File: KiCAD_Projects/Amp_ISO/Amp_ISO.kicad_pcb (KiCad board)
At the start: 2 copper layers, 0 parts

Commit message: MDver4.0だいたいできた｡絶縁アンプ基板作った｡
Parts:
- added C1: 0.1u, RP_KiCAD_Libs:C1608_WP, B.Cu at (11.5, 6.50)
- added C2: 0.1u, RP_KiCAD_Libs:C1608_WP, B.Cu at (23.0, 4.00)
- added D1: LED, RP_KiCAD_Libs:C1608_WP, B.Cu at (13.0, 13.5)
- added D2: LED, RP_KiCAD_Libs:C1608_WP, B.Cu at (21.0, 13.5)
- added P1: CONN_01X01, Connect:PINTST, F.Cu at (9.00, 11.5)
- added P2: CONN_01X03, RP_KiCAD_Connector:XA_3LC, F.Cu at (21.0, 7.50)
- added P3: CONN_01X01, Connect:PINTST, F.Cu at (8.00, 4.00)
- added P4: CONN_01X01, Connect:PINTST, F.Cu at (8.00, 6.50)
- added PC1: TLP117, RP_KiCAD_Libs:SOIC-5_3.9x4.9mm_Pitch1.27mm, B.Cu at (15.0, 2.50)
- added Q1: MOSFET_N, TO_SOT_Packages_SMD:SOT-23_Handsoldering, B.Cu at (13.0, 9.00)
- added R1: R, RP_KiCAD_Libs:C1608_WP, B.Cu at (9.00, 9.00)
- added R2: R, RP_KiCAD_Libs:C1608_WP, B.Cu at (9.50, 13.5)
- added R3: R, RP_KiCAD_Libs:C1608_WP, B.Cu at (17.5, 13.5)
- added R4: R, RP_KiCAD_Libs:C1608_WP, B.Cu at (14.5, 6.50)
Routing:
- net /GND_POWER: track 0.00 -> 20.5 mm
- net /5V_POWER: track 0.00 -> 20.4 mm
- net /5V_LOGIC: track 0.00 -> 14.7 mm
- net /GND_LOGIC: track 0.00 -> 12.9 mm
- net /SIGNAL_POWER: track 0.00 -> 6.82 mm
- net Net-(PC1-Pad3): track 0.00 -> 5.81 mm
- net /SIGNAL_LOGIC: track 0.00 -> 4.12 mm
- net Net-(D2-Pad2): track 0.00 -> 1.70 mm
- net Net-(D1-Pad2): track 0.00 -> 1.70 mm
- net Net-(Q1-PadD): track 0.00 -> 1.60 mm
- added copper zone on B.Cu, net (none)
- added copper zone on B.Cu, net /5V_LOGIC
- added copper zone on B.Cu, net /GND_LOGIC
- added copper zone on B.Cu, net /SIGNAL_LOGIC
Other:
- board outline added: 30 x 15 mm

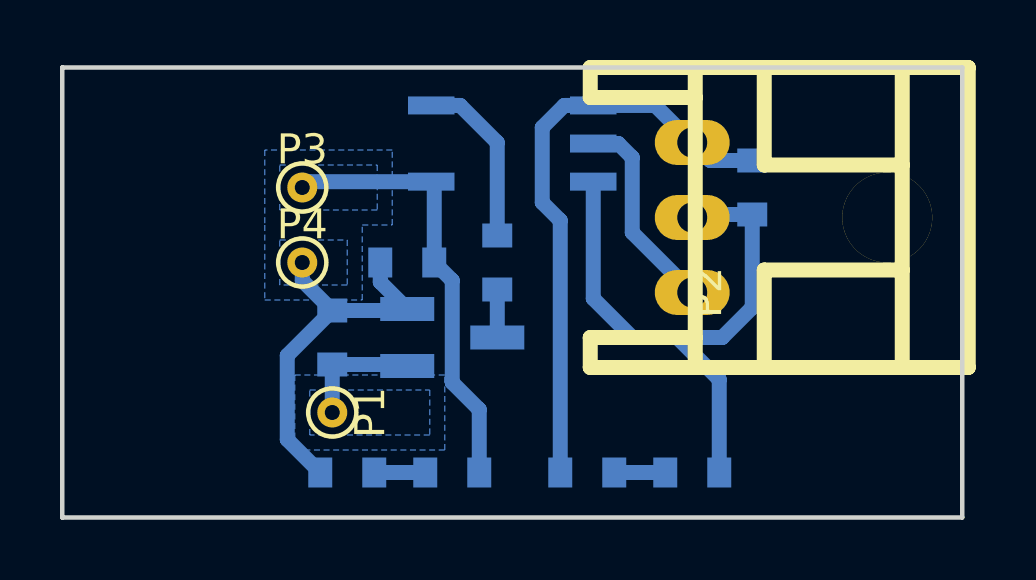
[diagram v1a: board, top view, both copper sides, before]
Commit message: 4.0発注かけた｡テレメトリとコンパネ作る
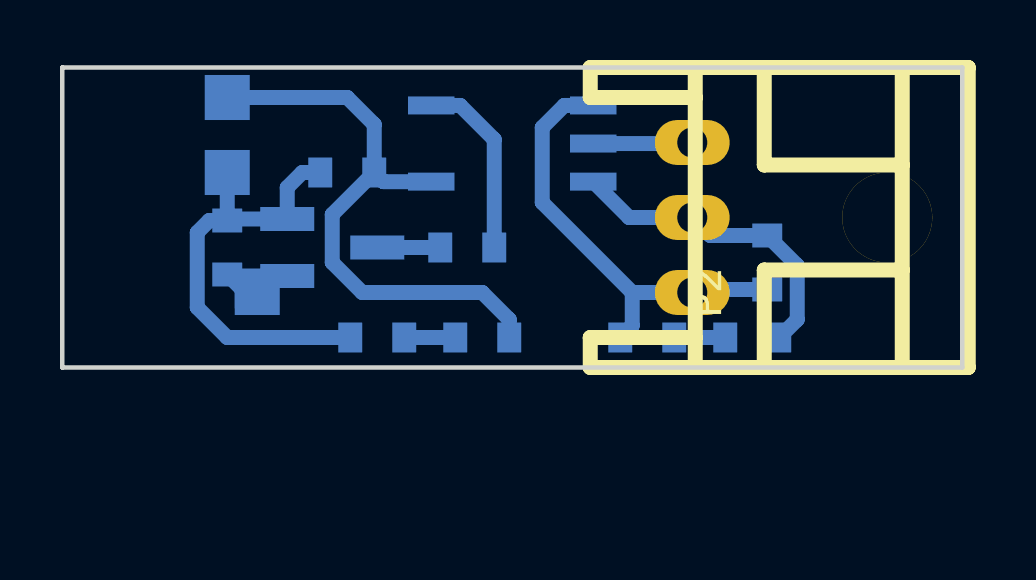
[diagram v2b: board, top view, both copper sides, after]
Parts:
- P1, P3, P4: footprint Connect:PINTST -> Measurement_Points:Measurement_Point_Square-SMD-Pad_Small; moved to B.Cu
- moved Q1 5.00 mm to (9.00, 6.00)
- moved D2 4.92 mm to (23.0, 9.00)
- moved R3 4.92 mm to (19.5, 9.00)
- moved P1 4.72 mm to (6.50, 7.50), turned to 90 degrees
- moved D1 4.61 mm to (14.0, 9.00)
- moved R2 4.61 mm to (10.5, 9.00)
- moved R1 4.61 mm to (5.50, 6.00)
- moved P3 3.91 mm to (5.50, 1.00)
- moved P4 3.91 mm to (5.50, 3.50)
- moved C1 3.61 mm to (9.50, 3.50)
- moved C2 2.55 mm to (23.5, 6.50), turned to 270 degrees
- moved R4 1.12 mm to (13.5, 6.00), turned to 180 degrees
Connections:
- P2 pad 1: /SIGNAL_POWER -> /GND_POWER
- P2 pad 3: /GND_POWER -> /SIGNAL_POWER
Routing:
- net /5V_POWER: track 20.4 -> 10.6 mm
- net /GND_POWER: track 20.5 -> 15.0 mm
- net /5V_LOGIC: track 14.7 -> 19.9 mm
- net /SIGNAL_POWER: track 6.82 -> 3.31 mm
- net /GND_LOGIC: track 12.9 -> 15.2 mm
- net /SIGNAL_LOGIC: track 4.12 -> 3.33 mm
- removed copper zone on B.Cu, net /5V_LOGIC
- removed copper zone on B.Cu, net /GND_LOGIC
- removed copper zone on B.Cu, net /SIGNAL_LOGIC
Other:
- board size 30 x 15 mm -> 30 x 10 mm
